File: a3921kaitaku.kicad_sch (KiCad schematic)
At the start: 42 parts, among them IC1 A3921KLPTR-T, J1 STlink, J2 CANport, M1 Motor_DC, Q1H NMOS, Q1L NMOS, Q2H NMOS, Q2L NMOS, U1 Si8640BA-B-IU, U2 STM32F303K8Tx, Y1 Crystal

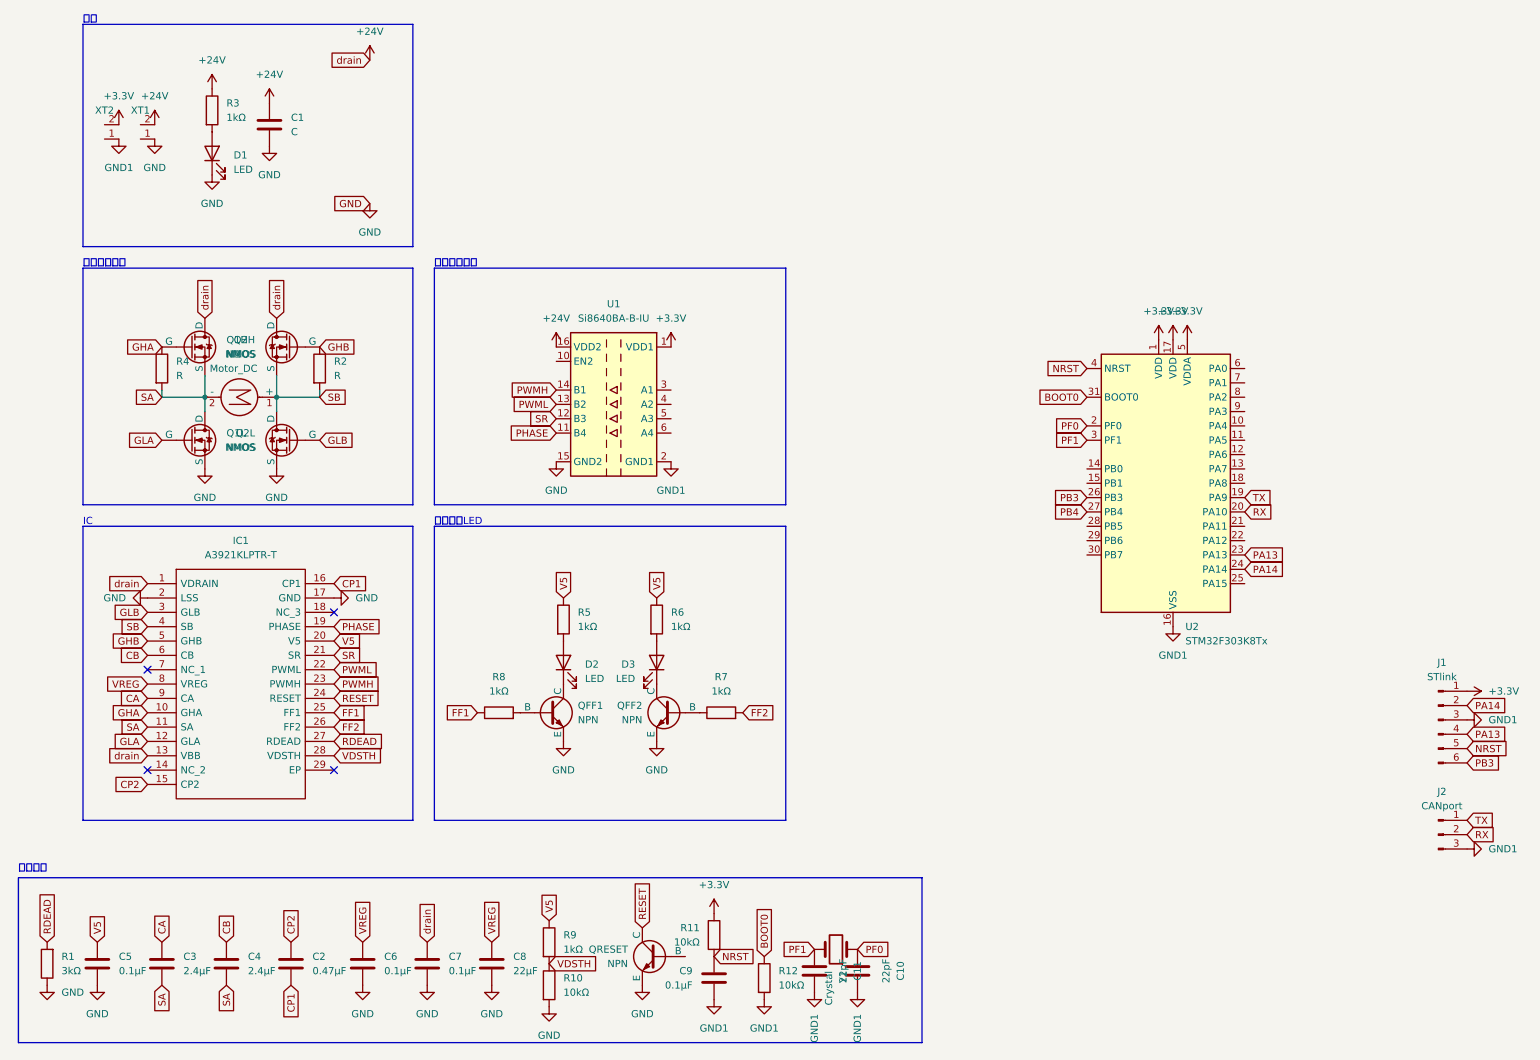
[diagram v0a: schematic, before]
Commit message: unti
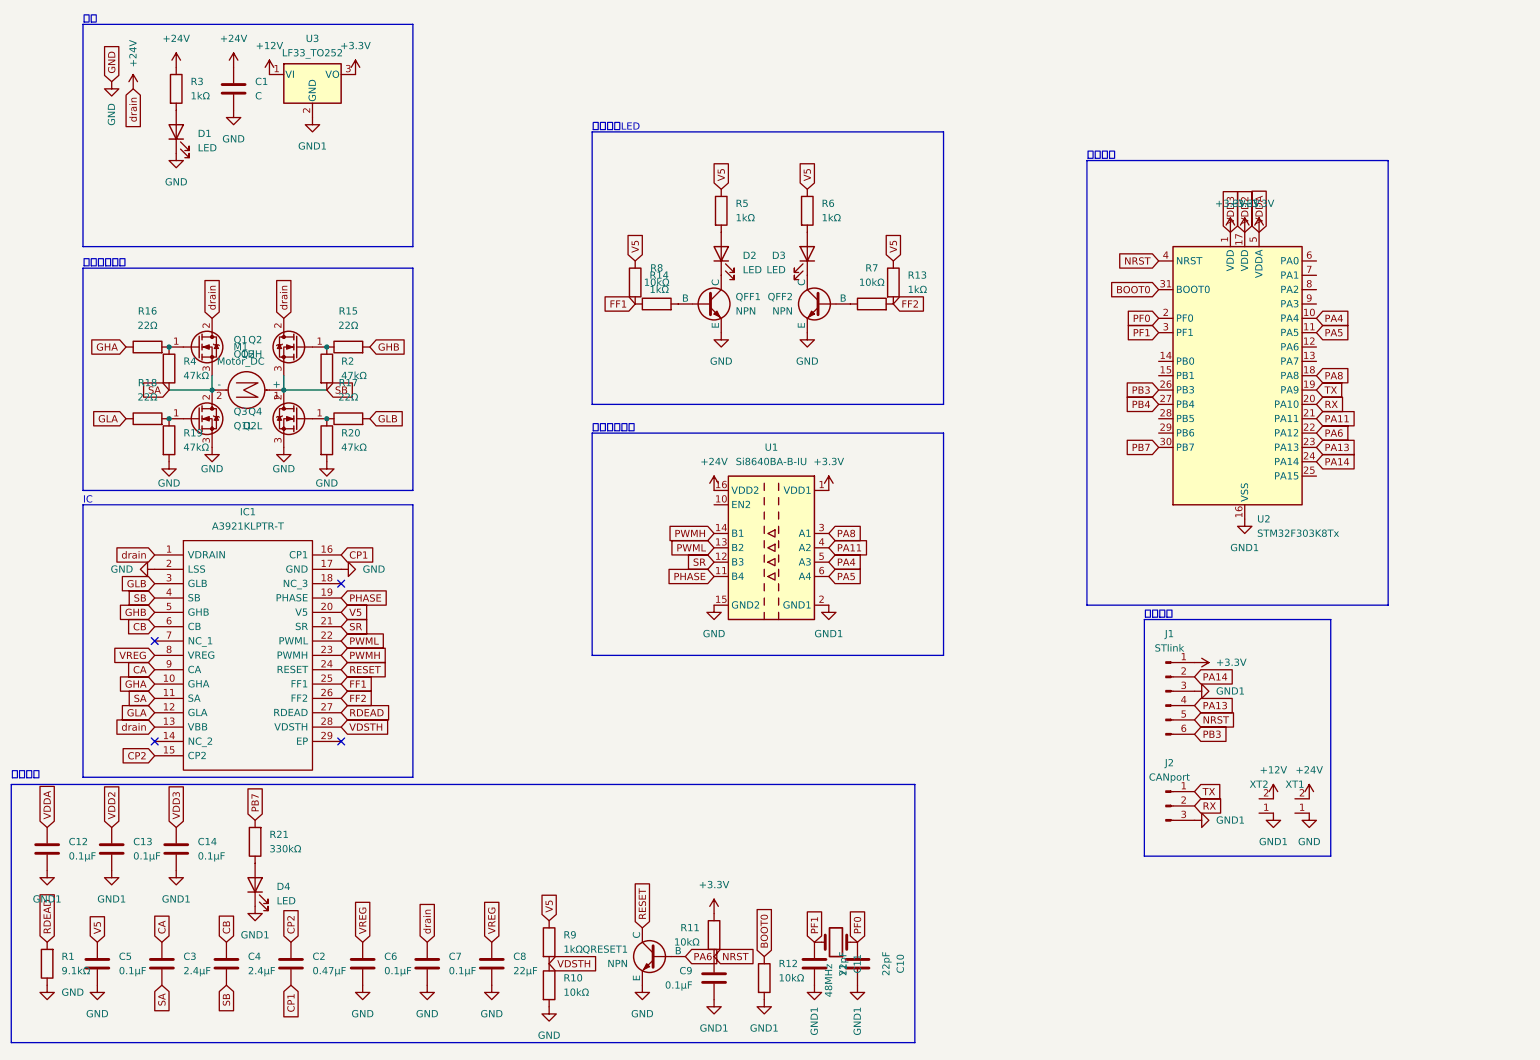
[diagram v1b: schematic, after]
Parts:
- removed Q1H, Q1L, Q2H, Q2L: NMOS, symbol Simulation_SPICE:NMOS
- added C12, C13, C14: 0.1μF, Capacitor_SMD:C_0603_1608Metric, symbol Device:C
- added D4: LED, LED_THT:LED_D3.0mm, symbol Device:LED
- added Q1: Q1H, Package_TO_SOT_SMD:TO-252-2, symbol Transistor_FET:QM6006D
- added Q2: Q2H, Package_TO_SOT_SMD:TO-252-2, symbol Transistor_FET:QM6006D
- added Q3: Q1L, Package_TO_SOT_SMD:TO-252-2, symbol Transistor_FET:QM6006D
- added Q4: Q2L, Package_TO_SOT_SMD:TO-252-2, symbol Transistor_FET:QM6006D
- added R13, R14: 1kΩ, Resistor_SMD:R_1206_3216Metric, symbol Device:R
- added R15, R16, R17, R18: 22Ω, Resistor_SMD:R_1206_3216Metric, symbol Device:R
- added R19, R20: 47kΩ, Resistor_SMD:R_1206_3216Metric, symbol Device:R
- added R21: 330kΩ, Resistor_SMD:R_1206_3216Metric, symbol Device:R
- added U3: LF33_TO252, Package_TO_SOT_SMD:TO-252-2, symbol Regulator_Linear:LF33_TO252
- IC1: footprint a3921:A3944KLPTRT -> Library:A3944KLPTRT
- J1: footprint (none) -> Connector_PinHeader_2.54mm:PinHeader_1x06_P2.54mm_Vertical
- J2: footprint (none) -> Connector_PinHeader_2.54mm:PinHeader_1x03_P2.54mm_Vertical
- M1: footprint Amass_XT60PW-M_footprints:Amass_XT60PW-M -> Library:Amass_XT60PW-M
- R1: value 3kΩ -> 9.1kΩ
- R2: value R -> 47kΩ
- R4: value R -> 47kΩ; footprint (none) -> Resistor_SMD:R_1206_3216Metric
- R5, R6: footprint (none) -> Resistor_SMD:R_1206_3216Metric
- R7, R8: value 1kΩ -> 10kΩ; footprint (none) -> Resistor_SMD:R_1206_3216Metric
- Y1: value Crystal -> 48MHz; footprint (none) -> Crystal:Crystal_HC49-U_Vertical
- renumbered QRESET to QRESET1
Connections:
- net +24V: now also Q1.2 (D), Q2.2 (D)
- net +3.3V: now also C12.1, C13.1, C14.1, U3.3 (VO); no longer XT2.2
- net FF1: now also R14.2
- net FF2: now also R13.2
- net GHA: now also R16.1; no longer R4.1
- net GHB: now also R15.2; no longer R2.1
- net GLA: now also R18.1
- net GLB: now also R17.2
- net GND: now also Q3.3 (S), Q4.3 (S), R19.2, R20.2
- net GND1: now also C12.2, C13.2, C14.2, D4.1 (K), U3.2 (GND)
- net SA: now also Q1.3 (S), Q3.2 (D); no longer C4.2
- net SB: now also C4.2, Q2.3 (S), Q4.2 (D)
- net V5: now also R13.1, R14.1
- net PA6: now reaches QRESET1.2 (B)
- net PA6: now also U2.22 (PA12)
- net PA4: now reaches U2.10 (PA4)
- net PA4: now also U1.5 (A3)
- net PA5: now reaches U2.11 (PA5)
- net PA5: now also U1.6 (A4)
- net PA8: now reaches U2.18 (PA8)
- net PA8: now also U1.3 (A1)
- net PA11: now reaches U2.21 (PA11)
- net PA11: now also U1.4 (A2)
- net PB7: now reaches U2.30 (PB7)
- net PB7: now also R21.2
- new net: Q4.1 (G), R17.1, R20.1
- new net: Q3.1 (G), R18.2, R19.1
- new net: Q1.1 (G), R16.2, R4.1
- new net: D4.2 (A), R21.1
- new net: Q2.1 (G), R15.1, R2.1
- new net +12V: U3.1 (VI), XT2.2
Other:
- note added: "コネクタ"
- note added: "マイコン"
- moved on the sheet: C1, C10, C11, D1, D2, D3, IC1, J1, J2, M1, QFF1, QFF2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
